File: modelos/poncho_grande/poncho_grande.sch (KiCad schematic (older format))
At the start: 0 parts

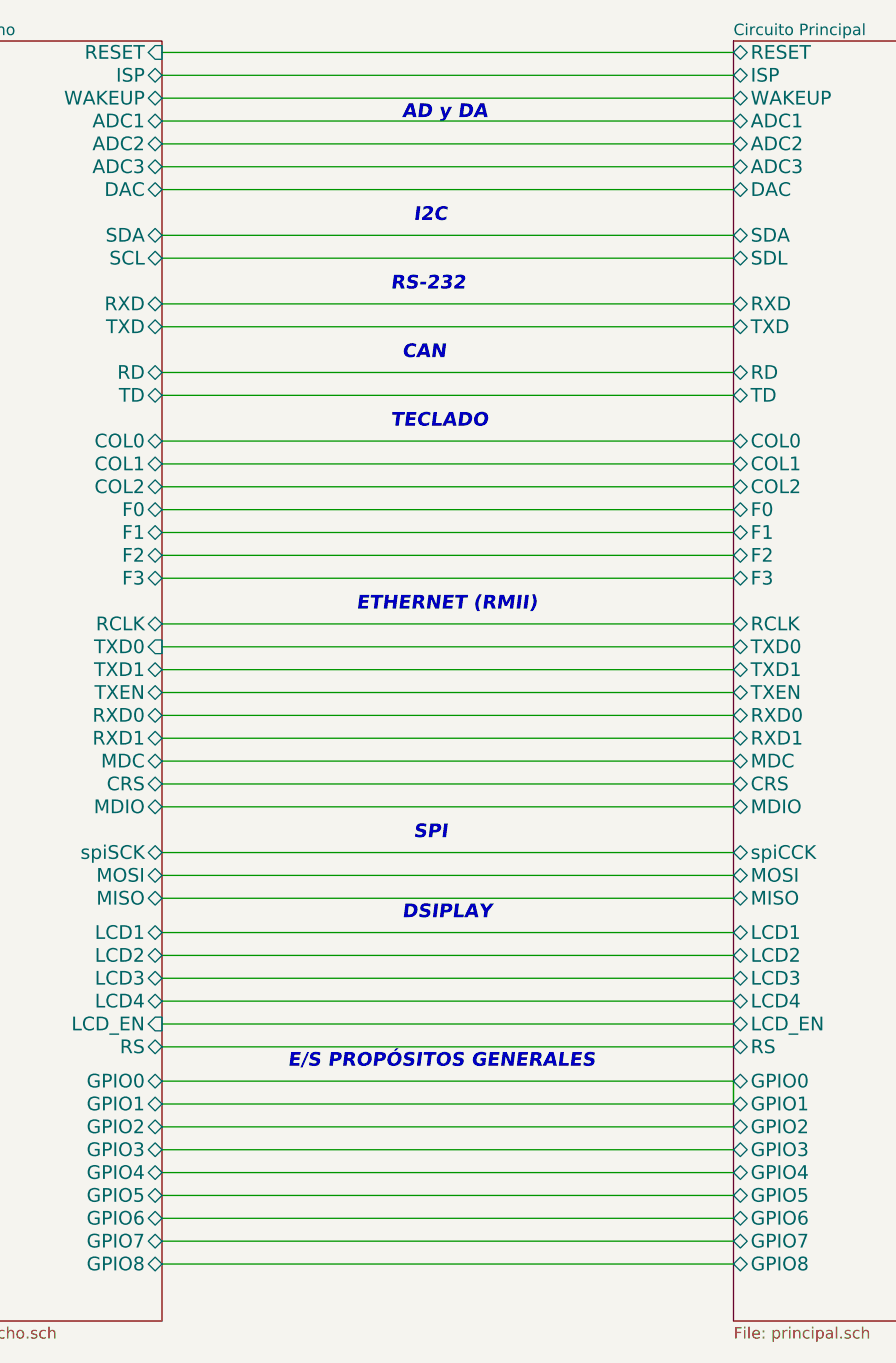
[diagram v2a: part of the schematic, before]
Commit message: * Mejoras y emprolijamiento en el esquemático y el PCB.
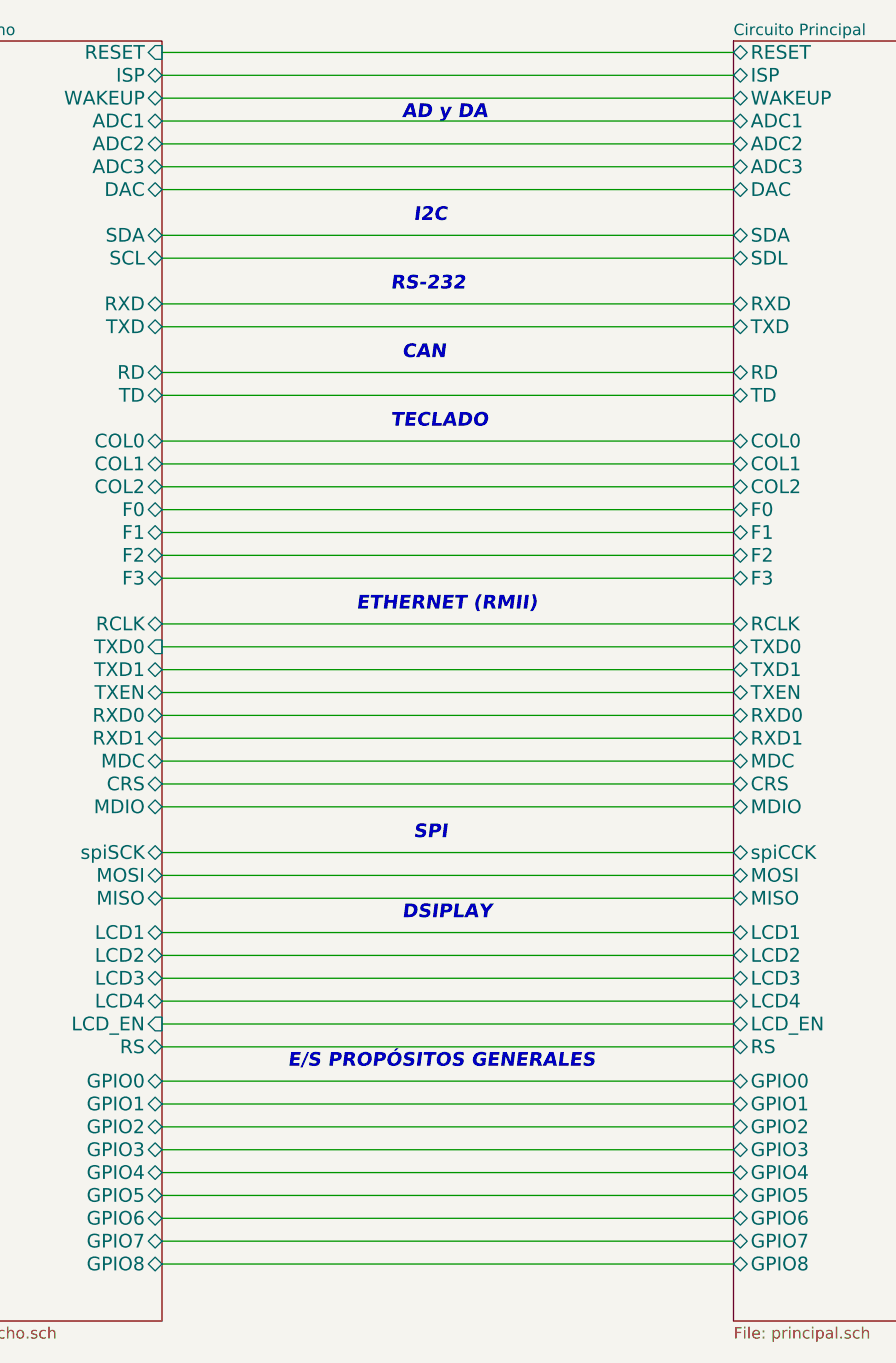
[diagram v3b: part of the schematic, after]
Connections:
- wire segments 48 -> 47
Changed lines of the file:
@@
 EESchema Schematic File Version 2
-LIBS:power
 LIBS:modelos_ponchos
-LIBS:conn
+LIBS:misc
+LIBS:poncho_grande-cache
 EELAYER 25 0
 EELAYER END
@@
 F 0 "#G1" H 9470 6400 60  0001 C CNN
 F 1 "OSHWA" H 9500 6303 60  0001 C CNN
-F 2 "" H 9500 6000 60  0000 C CNN
+F 2 "mod:OSHWA" H 9500 6000 60  0001 C CNN
 F 3 "" H 9500 6000 60  0000 C CNN
 	1    9500 6000
@@
 F 0 "#G2" H 10400 5497 60  0001 C CNN
 F 1 "LOGO" H 10400 6303 60  0001 C CNN
-F 2 "" H 10400 5900 60  0000 C CNN
+F 2 "mod:LOGO" H 10400 5900 60  0001 C CNN
 F 3 "" H 10400 5900 60  0000 C CNN
 	1    10400 5900
@@
 F36 "LCD_EN" B L 5250 5500 60
 F37 "RS" B L 5250 5600 60
-F38 "GPIO0" B L 5250 5750 60
-F39 "GPIO1" B L 5250 5850 60
-F40 "GPIO2" B L 5250 5950 60
-F41 "GPIO3" B L 5250 6050 60
-F42 "GPIO4" B L 5250 6150 60
-F43 "GPIO5" B L 5250 6250 60
-F44 "GPIO6" B L 5250 6350 60
-F45 "GPIO7" B L 5250 6450 60
-F46 "GPIO8" B L 5250 6550 60
-F47 "COL2" B L 5250 3150 60
-F48 "WAKEUP" B L 5250 1450 60
+F38 "GPIO2" B L 5250 5950 60
+F39 "GPIO3" B L 5250 6050 60
+F40 "GPIO4" B L 5250 6150 60
+F41 "GPIO5" B L 5250 6250 60
+F42 "GPIO6" B L 5250 6350 60
+F43 "GPIO7" B L 5250 6450 60
+F44 "GPIO8" B L 5250 6550 60
+F45 "COL2" B L 5250 3150 60
+F46 "WAKEUP" B L 5250 1450 60
+F47 "GPIO1" B L 5250 5850 60
+F48 "GPIO0" B L 5250 5750 60
 $EndSheet
 $Sheet
@@
 F48 "WAKEUP" B R 2750 1450 60
 $EndSheet
-Wire Wire Line
-	5250 3050 2750 3050
-Wire Wire Line
-	2750 3150 5250 3150
-Wire Wire Line
-	5250 3250 2750 3250
-Wire Wire Line
-	2750 3350 5250 3350
-Wire Wire Line
-	5250 3450 2750 3450
-Wire Wire Line
-	2750 3550 5250 3550
-Wire Wire Line
-	2750 3750 5250 3750
-Wire Wire Line
-	5250 3850 2750 3850
-Wire Wire Line
-	2750 3950 5250 3950
-Wire Wire Line
-	5250 4050 2750 4050
-Wire Wire Line
-	2750 4150 5250 4150
-Wire Wire Line
-	5250 4250 2750 4250
-Wire Wire Line
-	2750 4350 5250 4350
-Wire Wire Line
-	5250 4450 2750 4450
-Wire Wire Line
-	2750 4550 5250 4550
-Wire Wire Line
-	5250 4750 2750 4750
-Wire Wire Line
-	2750 4850 5250 4850
-Wire Wire Line
-	5250 4950 2750 4950
-Wire Wire Line
-	2750 5100 5250 5100
-Wire Wire Line
-	5250 5200 2750 5200
-Wire Wire Line
-	2750 5300 5250 5300
-Wire Wire Line
-	5250 5400 2750 5400
-Wire Wire Line
-	2750 5500 5250 5500
-Wire Wire Line
-	5250 5600 2750 5600
-Wire Wire Line
-	2750 5750 5250 5750
-Wire Wire Line
-	5250 5750 5250 5850
-Wire Wire Line
-	5250 5850 2750 5850
-Wire Wire Line
-	2750 5950 5250 5950
-Wire Wire Line
-	5250 6050 2750 6050
-Wire Wire Line
-	2750 6150 5250 6150
-Wire Wire Line
-	2750 6250 5250 6250
-Wire Wire Line
-	2750 6350 5250 6350
-Wire Wire Line
-	5250 6450 2750 6450
-Wire Wire Line
-	2750 6550 5250 6550
 Text Notes 3800 1550 0    60   Italic 12
 AD y DA
@@
 E/S PROPÓSITOS GENERALES
 Wire Wire Line
+	5250 6550 2750 6550
+Wire Wire Line
+	2750 6450 5250 6450
+Wire Wire Line
+	5250 6350 2750 6350
+Wire Wire Line
+	2750 6250 5250 6250
+Wire Wire Line
+	5250 6150 2750 6150
+Wire Wire Line
+	2750 6050 5250 6050
+Wire Wire Line
+	5250 5950 2750 5950
+Wire Wire Line
+	5250 5850 2750 5850
+Wire Wire Line
+	2750 5750 5250 5750
+Wire Wire Line
+	5250 5600 2750 5600
+Wire Wire Line
+	2750 5500 5250 5500
+Wire Wire Line
+	5250 5400 2750 5400
+Wire Wire Line
+	2750 5300 5250 5300
+Wire Wire Line
+	5250 5200 2750 5200
+Wire Wire Line
+	2750 5100 5250 5100
+Wire Wire Line
+	5250 4950 2750 4950
+Wire Wire Line
+	2750 4850 5250 4850
+Wire Wire Line
+	5250 4750 2750 4750
+Wire Wire Line
+	2750 4550 5250 4550
+Wire Wire Line
+	5250 4450 2750 4450
+Wire Wire Line
+	5250 4350 2750 4350
+Wire Wire Line
+	2750 4250 5250 4250
+Wire Wire Line
+	5250 4150 2750 4150
+Wire Wire Line
+	2750 4050 5250 4050
+Wire Wire Line
+	5250 3950 2750 3950
+Wire Wire Line
+	2750 3850 5250 3850
+Wire Wire Line
+	5250 3750 2750 3750
+Wire Wire Line
+	2750 3550 5250 3550
+Wire Wire Line
+	5250 3450 2750 3450
+Wire Wire Line
+	2750 3350 5250 3350
+Wire Wire Line
+	5250 3250 2750 3250
+Wire Wire Line
+	2750 3150 5250 3150
+Wire Wire Line
+	5250 3050 2750 3050
+Wire Wire Line
 	2750 2950 5250 2950
 Wire Wire Line
@@
 	2750 2350 5250 2350
 Wire Wire Line
-	5250 2150 2750 2150
-Wire Wire Line
-	2750 2050 5250 2050
-Wire Wire Line
-	5250 1850 2750 1850
-Wire Wire Line
-	2750 1750 5250 1750
-Wire Wire Line
-	5250 1650 2750 1650
-Wire Wire Line
-	2750 1550 5250 1550
+	2750 2150 5250 2150
+Wire Wire Line
+	5250 2050 2750 2050
+Wire Wire Line
+	2750 1850 5250 1850
+Wire Wire Line
+	5250 1750 2750 1750
+Wire Wire Line
+	2750 1650 5250 1650
+Wire Wire Line
+	5250 1550 2750 1550
 Wire Wire Line
 	2750 1450 5250 1450

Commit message: * Cambios en el esquemático. Ejemplo de Poncho simple con área para prototipado.
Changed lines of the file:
@@
 LIBS:modelos_ponchos
 LIBS:misc
+LIBS:conn
+LIBS:poncho_grande-cache
 EELAYER 25 0
 EELAYER END
@@
 $EndDescr
 $Comp
-L OSHWA #G1
+L OSHWA #G2
 U 1 1 560A0A28
-P 9500 6000
-F 0 "#G1" H 9470 6400 60  0001 C CNN
-F 1 "OSHWA" H 9500 6303 60  0001 C CNN
-F 2 "mod:OSHWA" H 9500 6000 60  0001 C CNN
-F 3 "" H 9500 6000 60  0000 C CNN
-	1    9500 6000
-	1    0    0    -1
-$EndComp
-$Comp
-L LOGO #G2
-U 1 1 560A0A3C
-P 10400 5900
-F 0 "#G2" H 10400 5497 60  0001 C CNN
-F 1 "LOGO" H 10400 6303 60  0001 C CNN
-F 2 "mod:LOGO" H 10400 5900 60  0001 C CNN
-F 3 "" H 10400 5900 60  0000 C CNN
-	1    10400 5900
+P 10800 6050
+F 0 "#G2" H 10770 6450 60  0001 C CNN
+F 1 "OSHWA" H 10800 6353 60  0001 C CNN
+F 2 "mod:OSHWA" H 10800 6050 60  0001 C CNN
+F 3 "" H 10800 6050 60  0000 C CNN
+	1    10800 6050
 	1    0    0    -1
 $EndComp
@@
 F7 "DAC" B L 5250 1850 60
 F8 "SDA" B L 5250 2050 60
-F9 "SDL" B L 5250 2150 60
+F9 "SCL" B L 5250 2150 60
 F10 "RXD" B L 5250 2350 60
 F11 "TXD" B L 5250 2450 60
@@
 Wire Wire Line
 	2750 1250 5250 1250
+$Comp
+L Logo_Poncho #G1
+U 1 1 560CFFC0
+P 10150 6000
+F 0 "#G1" H 10100 5600 60  0001 C CNN
+F 1 "Logo_Poncho" H 10350 5600 60  0001 C CNN
+F 2 "" H 10150 6000 60  0000 C CNN
+F 3 "" H 10150 6000 60  0000 C CNN
+	1    10150 6000
+	1    0    0    -1
+$EndComp
 $EndSCHEMATC
